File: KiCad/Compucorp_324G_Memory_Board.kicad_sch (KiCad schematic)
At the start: 12 parts, among them J10 Memory Interboard, U10 2102, U11 2102, U12 2102, U13 93L00, U14 93L00, U15 93L00, U9 2102

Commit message: Memory board updates
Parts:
- added D10, D11, D12, D9: D, symbol Device:D
- added Q1, Q2, Q3, Q4: 2N4403, symbol Simulation_SPICE:PNP
- added R16, R21, R24, R27: 3.3KΩ, symbol Device:R
- added R17, R20, R23, R26: 1KΩ, symbol Device:R
- added R18, R19, R22, R25: 10KΩ, symbol Device:R
- added U16: 74L75, symbol 74xx:74LS75
- added U17: TMC1871 (TCL03), symbol Compucorp_324G_Scientist:TMC1871
- added U18: 8KR11A, symbol Compucorp_324G_Scientist:ROM
- added U19: 8KR029, symbol Compucorp_324G_Scientist:ROM
- added U20: 8KR218, symbol Compucorp_324G_Scientist:ROM
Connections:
- net +5V: now also Q1.3 (E), Q2.3 (E), Q3.3 (E), Q4.3 (E), R17.2, R20.2, R23.2, R26.2, U16.5 (VCC), U17.1 (Pin_1), U18.1, U19.1, U20.1
- net GND: now also D10.2 (A), D11.2 (A), D12.2 (A), D9.2 (A), U16.12 (GND)
- net TCL03_24: now reaches U14.4 (P0)
- net TCL03_24: now also U17.24 (Pin_24), U18.11, U19.11, U20.11
- net TCL03_25: now reaches U14.5 (P1)
- net TCL03_25: now also U17.25 (Pin_25), U18.10, U19.10, U20.10
- net TCL03_26: now reaches U14.6 (P2)
- net TCL03_26: now also U17.26 (Pin_26), U18.9, U19.9, U20.9
- net TCL03_21: now reaches U14.7 (P3)
- net TCL03_21: now also U17.21 (Pin_21)
- net RAM_D_{IN1}: now reaches U9.11 (D_{IN})
- net RAM_D_{IN1}: now also U16.8 (~{Q3})
- net RAM_D_{OUT1}: now reaches U9.12 (D_{OUT})
- net RAM_D_{OUT1}: now also R21.1
- net TCL03_28: now reaches U13.4 (P0)
- net TCL03_28: now also U17.28 (Pin_28), U18.7, U19.7, U20.7
- net TCL03_29: now reaches U13.5 (P1)
- net TCL03_29: now also U17.29 (Pin_29), U18.6, U19.6, U20.6
- net TCL03_30: now reaches U13.6 (P2)
- net TCL03_30: now also U17.30 (Pin_30), U18.5, U19.5, U20.5
- net TCL03_08: now reaches U13.7 (P3)
- net TCL03_08: now also U17.8 (Pin_8), U18.4, U19.4, U20.4
- net IB_10: now reaches J10.a10 (Pin_a10)
- net IB_10: now also R18.1, U18.21, U19.21, U20.21
- net IB_02: now reaches J10.a2 (Pin_a2)
- net IB_02: now also U17.3 (Pin_3)
- net IB_28: now reaches J10.a28 (Pin_a28)
- net IB_28: now also U16.2 (D0)
- net IB_29: now reaches J10.a29 (Pin_a29)
- net IB_29: now also U16.3 (D1)
- net IB_30: now reaches J10.a30 (Pin_a30)
- net IB_30: now also U16.6 (D2)
- net IB_31: now reaches J10.a31 (Pin_a31)
- net IB_31: now also U16.7 (D3)
- net IB_33: now reaches J10.a33 (Pin_a33)
- net IB_33: now also J10.b33 (Pin_b33), U16.13 (E01), U16.4 (E23)
- net -25V: now reaches J10.a36 (Pin_a36)
- net -25V: now also J10.b36 (Pin_b36), U18.19, U19.19, U20.19
- net IB_40: now reaches J10.a40 (Pin_a40)
- net IB_40: now also U17.2 (Pin_2)
- net IB_07: now reaches J10.a7 (Pin_a7)
- net IB_07: now also R25.1, U18.22, U19.22, U20.22
- net IB_08: now reaches J10.a8 (Pin_a8)
- net IB_08: now also R22.1, U18.23, U19.23, U20.23
- net IB_09: now reaches J10.a9 (Pin_a9)
- net IB_09: now also R19.1, U18.20, U19.20, U20.20
- net IB_23: now reaches J10.b23 (Pin_b23)
- net IB_23: now also U18.3, U19.3, U20.3
- net RAM_D_{IN2}: now reaches U10.11 (D_{IN})
- net RAM_D_{IN2}: now also U16.11 (~{Q2})
- net RAM_D_{OUT2}: now reaches U10.12 (D_{OUT})
- net RAM_D_{OUT2}: now also R16.1
- net RAM_D_{IN3}: now reaches U11.11 (D_{IN})
- net RAM_D_{IN3}: now also U16.14 (~{Q1})
- net RAM_D_{OUT3}: now reaches U11.12 (D_{OUT})
- net RAM_D_{OUT3}: now also R27.1
- net RAM_D_{IN4}: now reaches U12.11 (D_{IN})
- net RAM_D_{IN4}: now also U16.1 (~{Q0})
- net RAM_D_{OUT4}: now reaches U12.12 (D_{OUT})
- net RAM_D_{OUT4}: now also R24.1
- net TCL03_11: now reaches U15.4 (P0)
- net TCL03_11: now also U17.11 (Pin_11)
- net TCL03_18: now reaches U15.5 (P1)
- net TCL03_18: now also U17.18 (Pin_18), U18.17, U19.17, U20.17
- net TCL03_23: now reaches U15.6 (P2)
- net TCL03_23: now also U17.23 (Pin_23), U18.12, U19.12, U20.12
- new net: D9.1 (K), Q2.1 (C), R18.2
- new net: Q3.2 (B), R23.1, R24.2
- new net: Q1.2 (B), R20.1, R21.2
- new net: Q4.2 (B), R26.1, R27.2
- new net: D10.1 (K), Q1.1 (C), R19.2
- new net: Q2.2 (B), R16.2, R17.1
- new net: D11.1 (K), Q3.1 (C), R22.2
- new net: D12.1 (K), Q4.1 (C), R25.2
- new net TCL03_09: U17.9 (Pin_9), U18.27, U19.27, U20.27
- new net TCL03_10: U17.10 (Pin_10), U18.26, U19.26, U20.26
- new net TCL03_13: U17.13 (Pin_13), U18.25, U19.25, U20.25
- new net TCL03_14: U17.14 (Pin_14), U18.24, U19.24, U20.24
- new net TCL03_16: U17.16 (Pin_16), U18.28, U19.28, U20.28
- new net TCL03_17: U17.17 (Pin_17), U18.18, U19.18, U20.18
- new net TCL03_19: U17.19 (Pin_19)
- new net TCL03_20: U17.20 (Pin_20)
- new net TCL03_27: U17.27 (Pin_27), U18.8, U19.8, U20.8
- new net TCL03_35: U17.35 (Pin_35), U18.2, U19.2, U20.2
- no-connect marks 41 -> 67
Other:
- note added: "Huh?"
- moved on the sheet: R15, R4, R5, R6

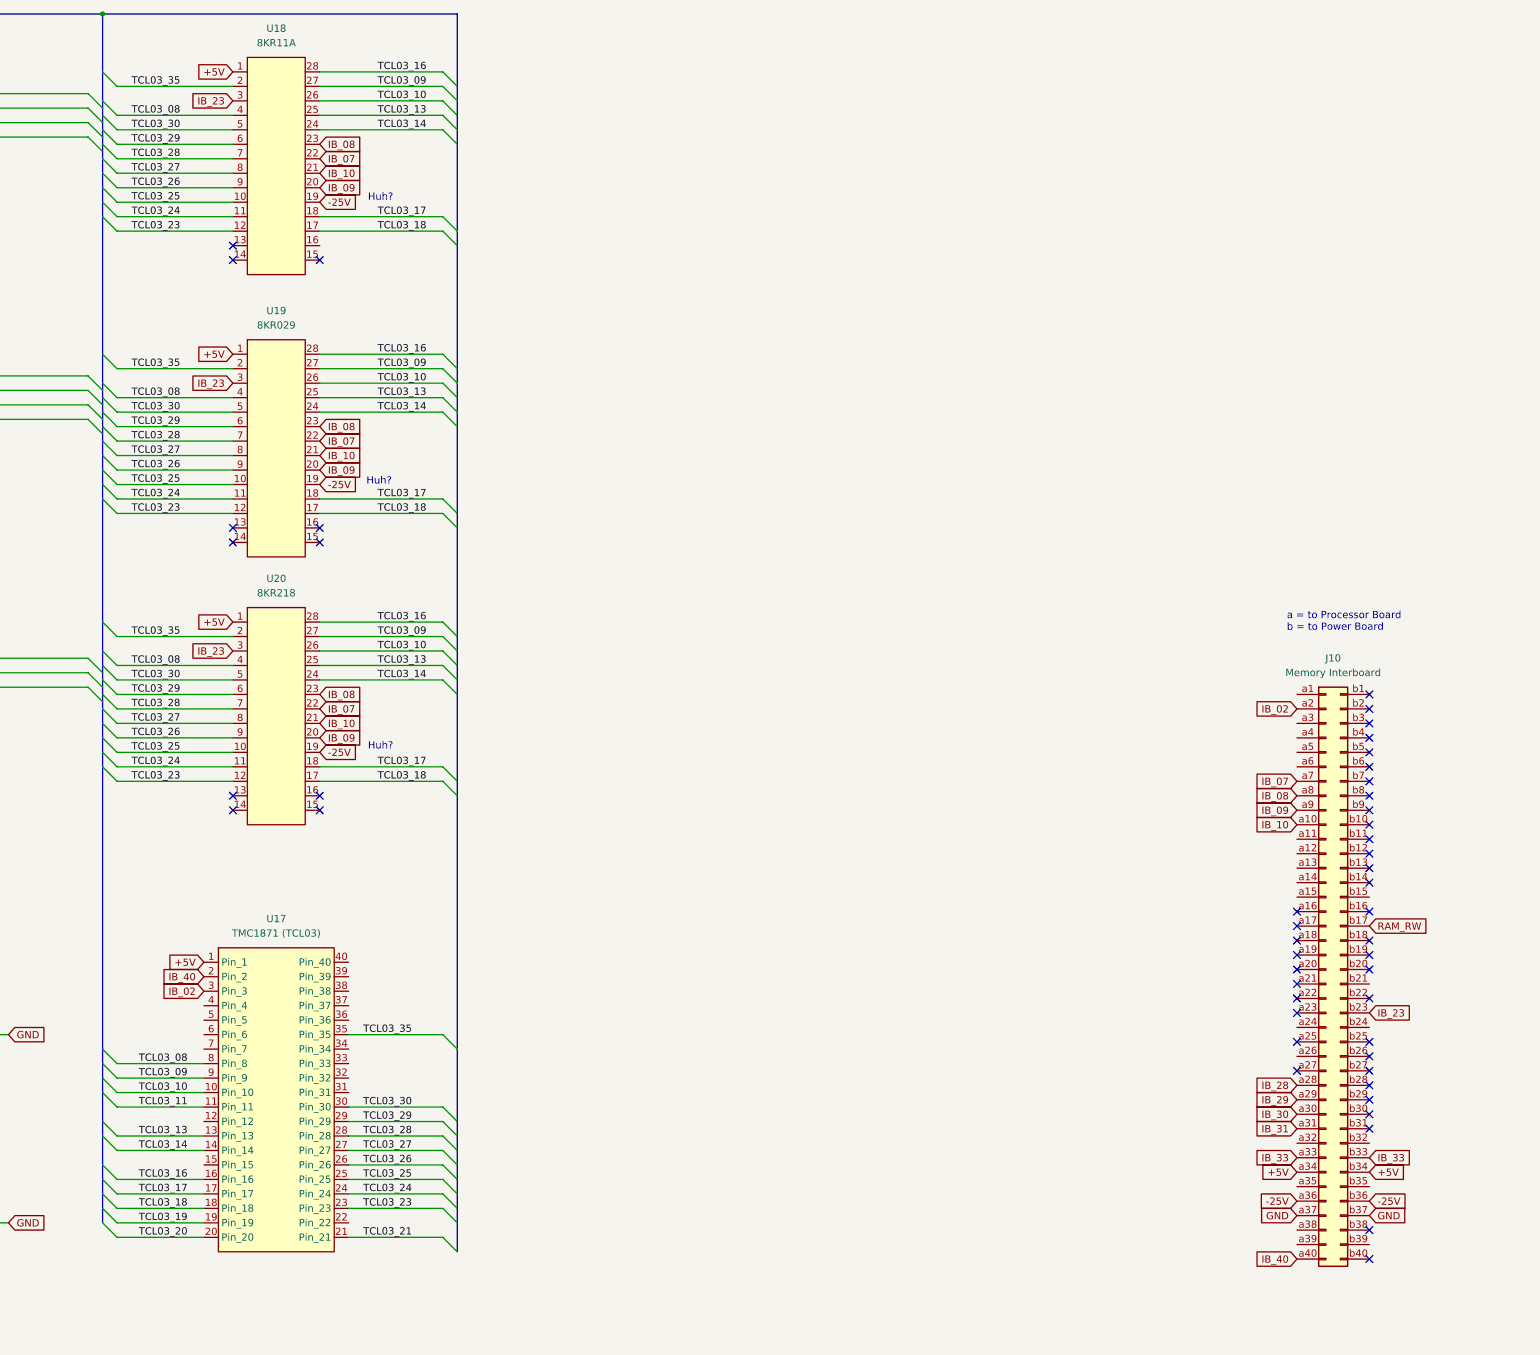
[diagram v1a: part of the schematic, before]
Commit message: Memory board updates
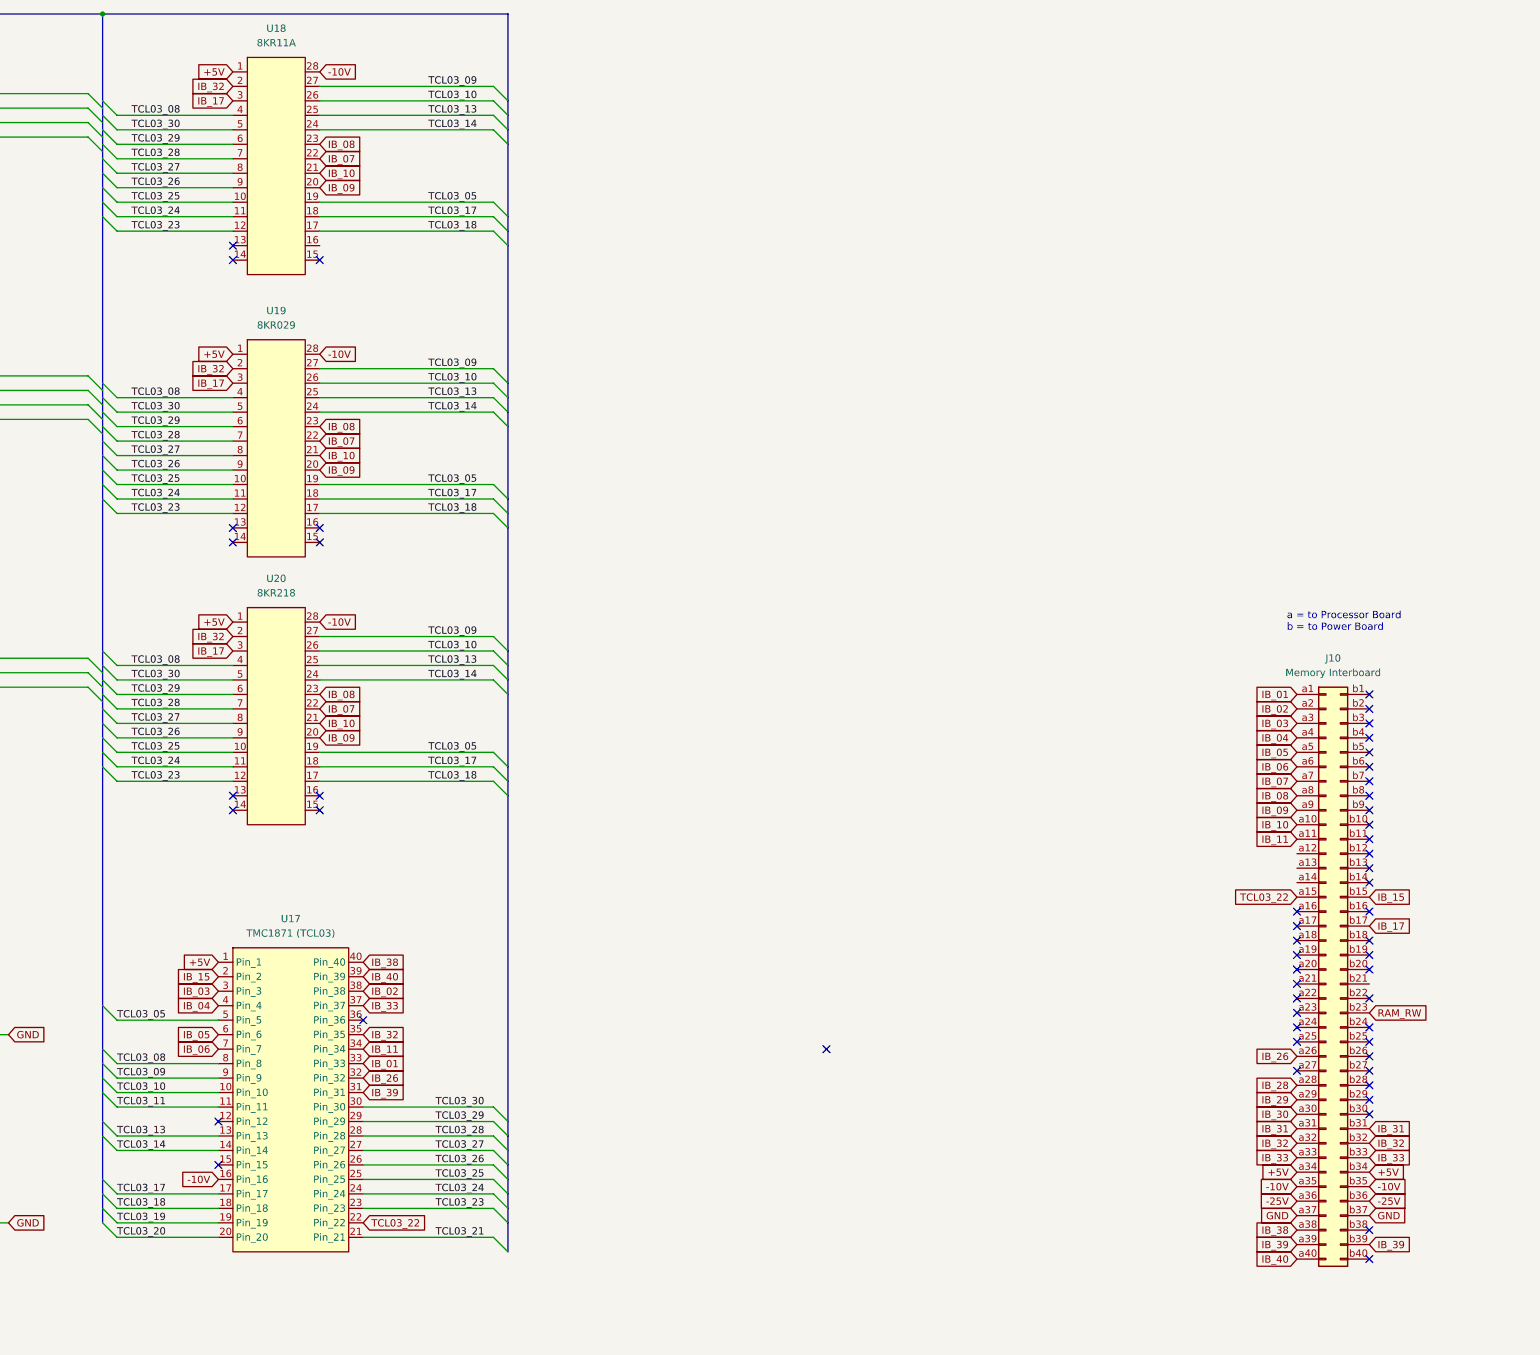
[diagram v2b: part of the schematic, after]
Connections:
- net TCL03_16 is gone; now on net -10V: U17.16 (Pin_16), U18.28, U19.28, U20.28
- net TCL03_35 is gone; now on net IB_32: U17.35 (Pin_35), U18.2, U19.2, U20.2
- net -25V: no longer U18.19, U19.19, U20.19
- net IB_02: now also U17.38 (Pin_38); no longer U17.3 (Pin_3)
- net IB_31: now also J10.b31 (Pin_b31)
- net IB_33: now also U17.37 (Pin_37)
- net IB_40: now also U17.39 (Pin_39); no longer U17.2 (Pin_2)
- net RAM_RW: now also J10.b23 (Pin_b23); no longer J10.b17 (Pin_b17)
- net IB_01: now reaches J10.a1 (Pin_a1)
- net IB_01: now also U17.33 (Pin_33)
- net IB_11: now reaches J10.a11 (Pin_a11)
- net IB_11: now also U17.34 (Pin_34)
- net TCL03_22: now reaches J10.a15 (Pin_a15)
- net TCL03_22: now also U17.22 (Pin_22)
- net IB_26: now reaches J10.a26 (Pin_a26)
- net IB_26: now also U17.32 (Pin_32)
- net IB_03: now reaches J10.a3 (Pin_a3)
- net IB_03: now also U17.3 (Pin_3)
- net IB_32: now reaches J10.a32 (Pin_a32)
- net IB_32: now also J10.b32 (Pin_b32)
- net -10V: now reaches J10.a35 (Pin_a35)
- net -10V: now also J10.b35 (Pin_b35)
- net IB_38: now reaches J10.a38 (Pin_a38)
- net IB_38: now also U17.40 (Pin_40)
- net IB_39: now reaches J10.a39 (Pin_a39)
- net IB_39: now also J10.b39 (Pin_b39), U17.31 (Pin_31)
- net IB_04: now reaches J10.a4 (Pin_a4)
- net IB_04: now also U17.4 (Pin_4)
- net IB_05: now reaches J10.a5 (Pin_a5)
- net IB_05: now also U17.6 (Pin_6)
- net IB_06: now reaches J10.a6 (Pin_a6)
- net IB_06: now also U17.7 (Pin_7)
- net IB_15: now reaches J10.b15 (Pin_b15)
- net IB_15: now also U17.2 (Pin_2)
- net TCL03_05: now reaches U17.5 (Pin_5)
- net TCL03_05: now also U18.19, U19.19, U20.19
- net IB_23 renamed IB_17
- net IB_17: now also J10.b17 (Pin_b17); no longer J10.b23 (Pin_b23)
- no-connect marks 67 -> 72
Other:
- note removed: "Huh?"
- moved on the sheet: U17
